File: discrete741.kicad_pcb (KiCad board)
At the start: 2 copper layers, 10.2 x 7.6 mm, 33 parts, among them J1 DIP-8 Pins, Q1 CET3904E, Q10 CET3904E, Q11 CET3904E, Q12 CET3906E, Q13 CET3906E, Q14 CET3904E, Q15 CET3904E, Q16 CET3904E, Q17 CET3904E, Q18 CET3904E, Q2 CET3904E, Q20 CET3906E, Q22 CET3904E, Q3 CET3906E, Q4 CET3906E, Q5 CET3904E, Q6 CET3904E, Q7 CET3904E, Q8 CET3906E, Q9 CET3906E

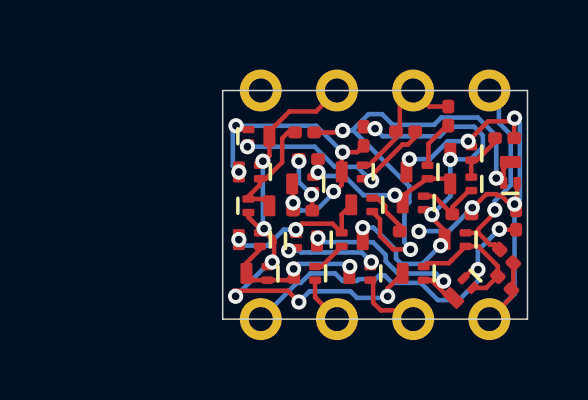
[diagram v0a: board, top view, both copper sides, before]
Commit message: cosmetic changes
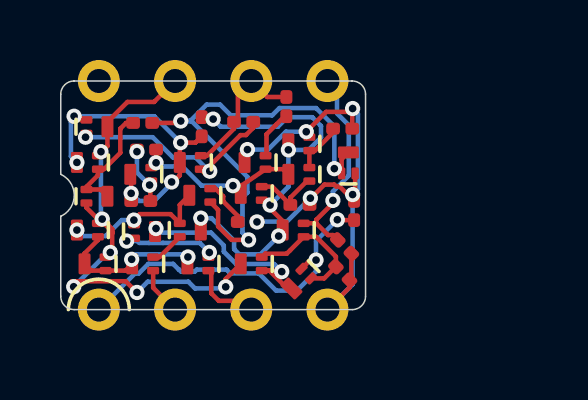
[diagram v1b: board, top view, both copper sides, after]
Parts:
- moved Q13 5.41 mm to (77.1, 71.3)
- moved Q16 5.41 mm to (82.5, 72.3)
- moved Q9 5.41 mm to (77.1, 73.5)
- moved R3 5.41 mm to (85.6, 75.0)
- moved J1 5.41 mm to (77.5, 76.2)
- moved Q10 5.41 mm to (80.8, 72.4)
- moved Q11 5.41 mm to (85.8, 71.3)
- moved Q12 5.41 mm to (77.4, 72.4)
- moved Q14 5.41 mm to (77.4, 70.1)
- moved Q2 5.41 mm to (78.9, 74.7)
- moved Q7 5.41 mm to (82.5, 74.7)
- moved R10 5.41 mm to (83.7, 69.4)
- moved R11 5.41 mm to (85.6, 70.2)
- moved R5 5.41 mm to (78.9, 70.0)
- moved Q15 5.41 mm to (80.5, 71.3)
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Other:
- outline, holes or cut-outs redrawn
- board text added: "MAGIC DORITO Discrete 741 DIP-8 ettingersam@gmail"
